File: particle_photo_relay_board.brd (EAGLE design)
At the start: 100 x 80 mm, 12 parts, among them Q1 600mA/40V

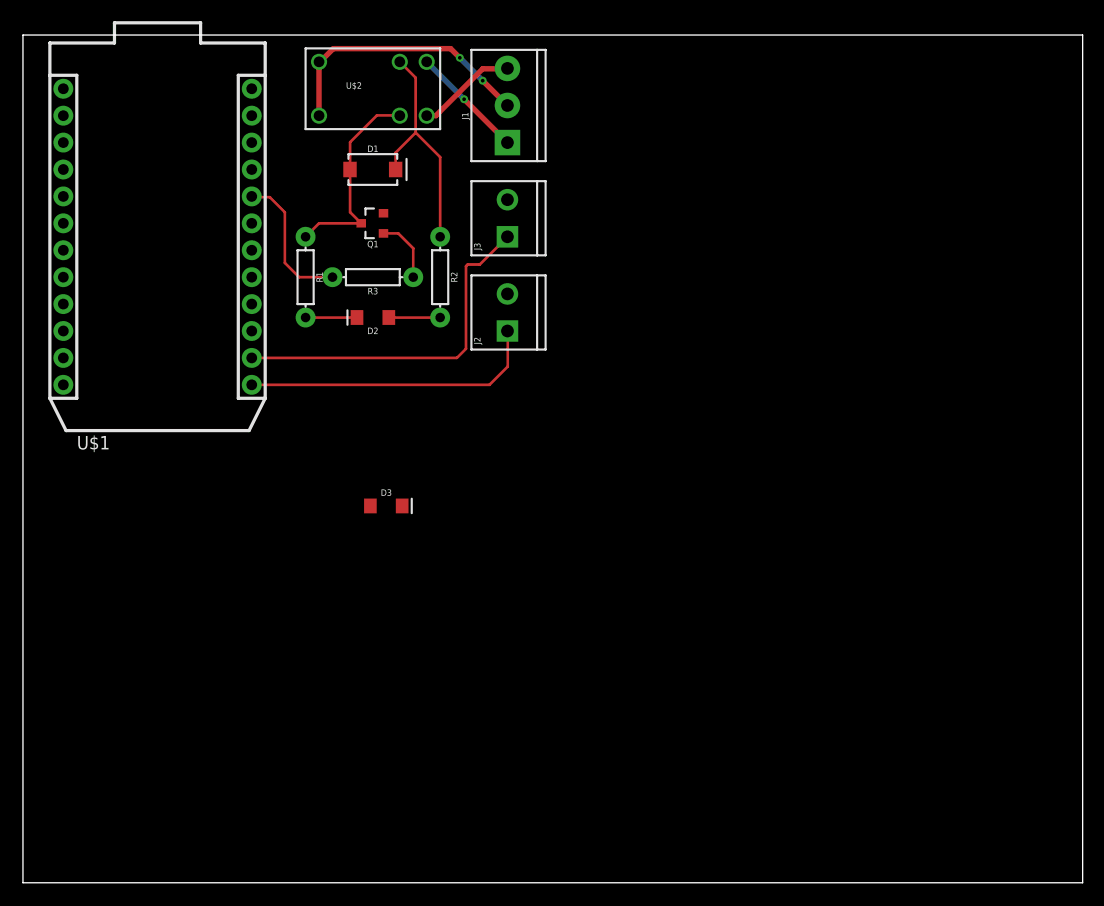
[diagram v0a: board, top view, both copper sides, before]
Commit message: Add files via upload
P.R.A.C.C REV1 SCH and BRD files ready for review.
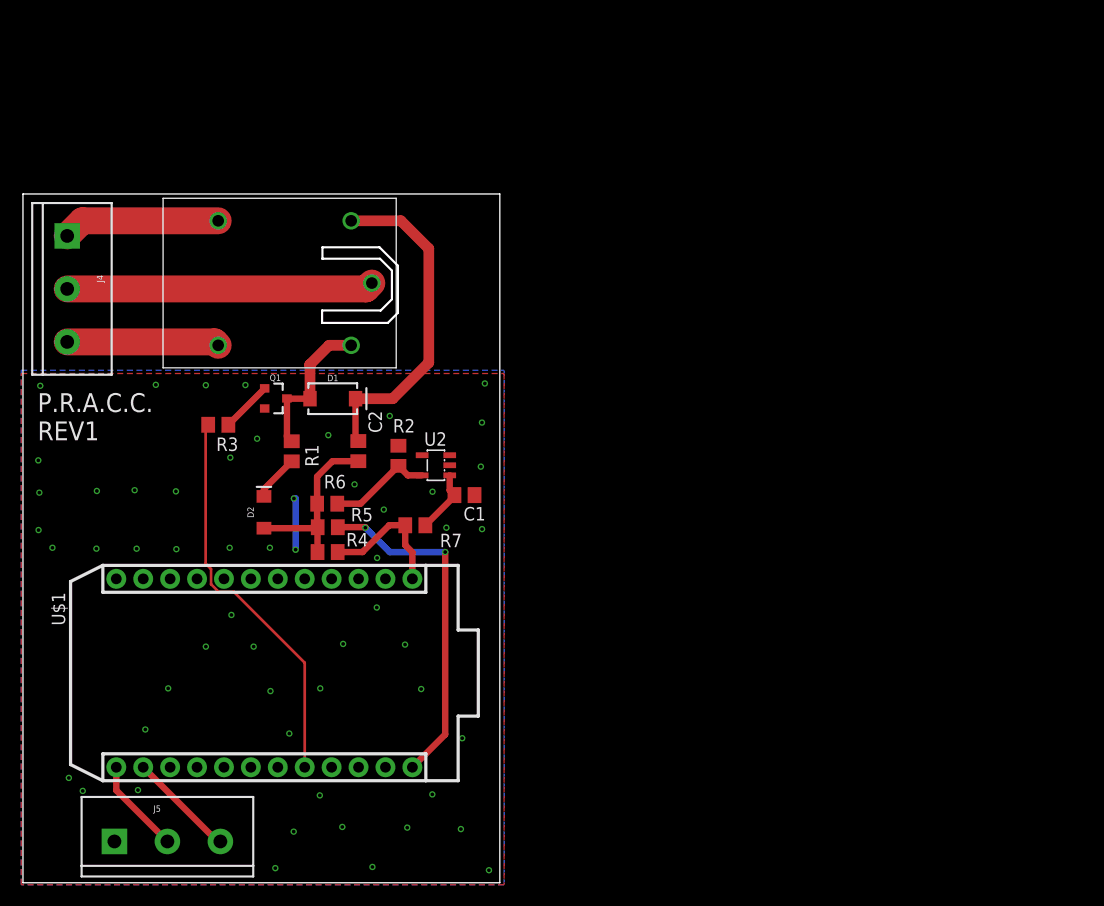
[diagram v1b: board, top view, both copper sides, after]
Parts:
- removed D3: GREEN, SparkFun-LED:LED-1206
- removed J1: (no value), SparkFun-Connectors:SCREWTERMINAL-3.5MM-3
- removed J2, J3: (no value), SparkFun-Retired:SCREWTERMINAL-3.5MM-2
- added C1, C2: 1uF, rcl:C0805
- added J4, J5: (no value), SparkFun-Connectors:SCREWTERMINAL-5MM-3
- added R4, R7: 0, rcl:R0805
- added R5, R6: 0 - DNI, rcl:R0805
- added U2: MIC5219BM5, v-reg-micrel:SOT23-5
- R1: value (none) -> 330; device SparkFun-Resistors:AXIAL-0.3 -> rcl:R0805
- R2, R3: value (none) -> 10; device SparkFun-Resistors:AXIAL-0.3 -> rcl:R0805
- U$2: value RELAY-SPDT-2-G5V -> RELAYOMRON; device SparkFun-Retired:RELAY-G5V -> Particle:G5LE-14-DC5
- moved D1 22.0 mm to (29.2, 45.7)
- moved D2 21.1 mm to (22.7, 35.0), turned to 90 degrees
- moved R3 20.2 mm to (18.4, 43.2)
- moved U$2 20.1 mm to (24.7, 56.6)
- moved Q1 18.9 mm to (23.8, 45.7), turned to 270 degrees
- moved R2 18.1 mm to (31.6, 40.7)
- moved R1 16.5 mm to (25.4, 40.7)
- moved U$1 12.0 mm to (3.73, 30.0), turned to 270 degrees
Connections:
- removed net 3V3: U$1.24
- removed net N$10: J3.1, U$1.14
- removed net N$5: R3.P$2, U$1.20
- removed net N$6: J2.1, U$1.13
- removed net N$7: J1.1, U$2.1
- removed net N$8: J1.3, U$2.10
- removed net N$9: J1.2, U$2.5, U$2.6
- removed net VCC: D2.A, R2.P$2
- removed net VIN: U$1.1
- new net 3V3_BACKUP: C2.1, R6.1, U2.5
- new net 3V3_PHOTON: R5.1, U$1.24
- new net COM: J4.2, U$2.COMMON
- new net NC: J4.3, U$2.CLOSED
- new net NO: J4.1, U$2.OPEN
- new net PHOTON_D0: J5.2, U$1.13
- new net PHOTON_D1: J5.3, U$1.14
- new net PHOTON_D7: R3.2, U$1.20
- new net VBUS_BACKUP: C1.1, R7.1, U2.1
- new net VCOIL: D2.A, R2.2, R4.2, R5.2, R6.2
- new net VIN_PHOTON: R4.1, R7.2, U$1.1
- net GND: now also C1.2, C2.2, J5.1, U2.2
- net N$1: now also R1.1, U$2.COIL2; no longer R1.P$1, U$2.9
- net N$2: now also R2.1, U$2.COIL1; no longer R2.P$1, U$2.2
- net N$3: now also R1.2; no longer R1.P$2
- net N$4: now also R3.1; no longer R3.P$1
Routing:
- net PHOTON_D7: track 0.00 -> 37.1 mm
- net N$10: track 33.4 -> 0.00 mm
- net 3V3_PHOTON: track 0.00 -> 32.7 mm, vias 0 -> 2
- net COM: track 0.00 -> 29.0 mm
- net N$6: track 28.2 -> 0.00 mm
- net N$9: track 25.6 -> 0.00 mm, vias 2 -> 0
- net VCOIL: track 0.00 -> 16.8 mm
- net NO: track 0.00 -> 14.8 mm
- net NC: track 0.00 -> 14.4 mm
- net N$5: track 13.6 -> 0.00 mm
- net VIN_PHOTON: track 0.00 -> 12.8 mm
- net N$7: track 10.8 -> 0.00 mm, vias 1 -> 0
- net PHOTON_D1: track 0.00 -> 10.2 mm
- net 3V3_BACKUP: track 0.00 -> 9.86 mm
- net N$8: track 9.47 -> 0.00 mm
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- added copper zone on layer 1, net GND
- added copper zone on layer 16, net GND
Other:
- board size 100 x 80 mm -> 45 x 65 mm
- board text added: "P.R.A.C.C."
- board text added: "REV1"
